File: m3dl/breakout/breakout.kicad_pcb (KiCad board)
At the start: 2 copper layers, 40 x 26 mm, 15 parts, among them J1 WEST TOP, J2 EAST TOP, J3 WEST BOT, J4 EAST BOT, J5 North, J6 South

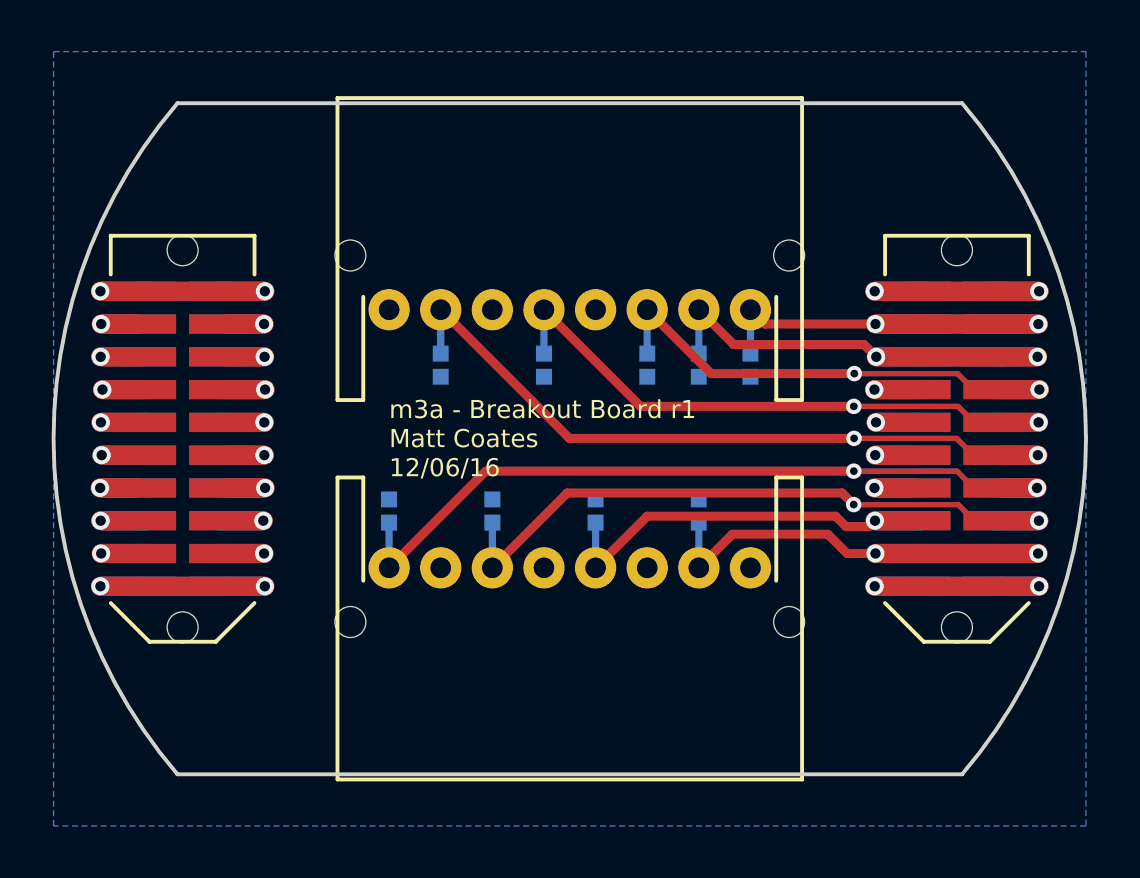
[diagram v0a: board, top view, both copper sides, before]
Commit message: Final Tweaks before manufacture
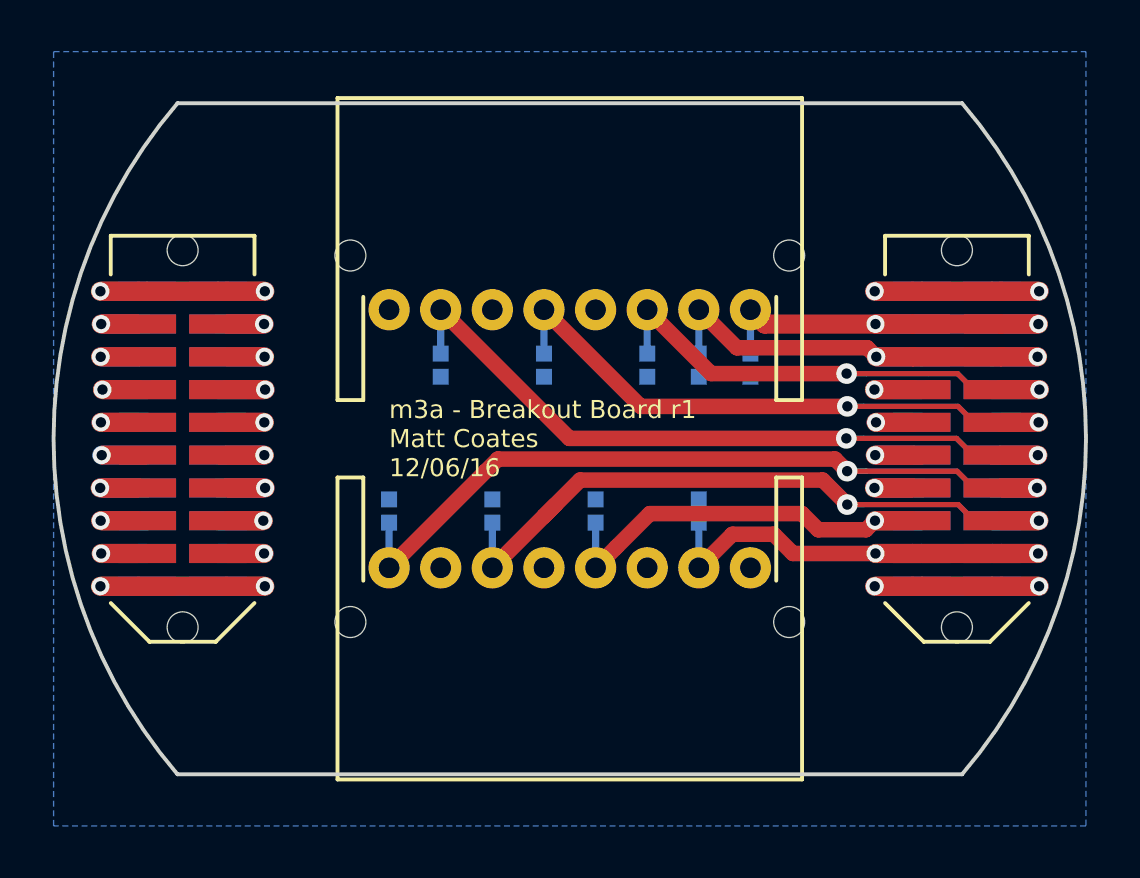
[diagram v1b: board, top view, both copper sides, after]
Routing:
- net /PWR: track 32.0 -> 33.7 mm
- net /PYRO4: track 36.0 -> 37.2 mm
- net /PYRO1: track 25.6 -> 26.4 mm
- net /PYRO3: track 34.6 -> 35.2 mm
- net /PYRO2: track 30.1 -> 30.7 mm
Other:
- net class Default: clearance 0.2 -> 0.15
- rule trace_clearance: 0.2 -> 0.15
